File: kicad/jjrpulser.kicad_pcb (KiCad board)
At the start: 2 copper layers, 51.1 x 44.7 mm, 18 parts, among them J1 3.3V, J2 3.3V, J3 Screw_Terminal_HOT, J4 Screw_Terminal_COLD, J5 Conn_UART, U1 ESP-12

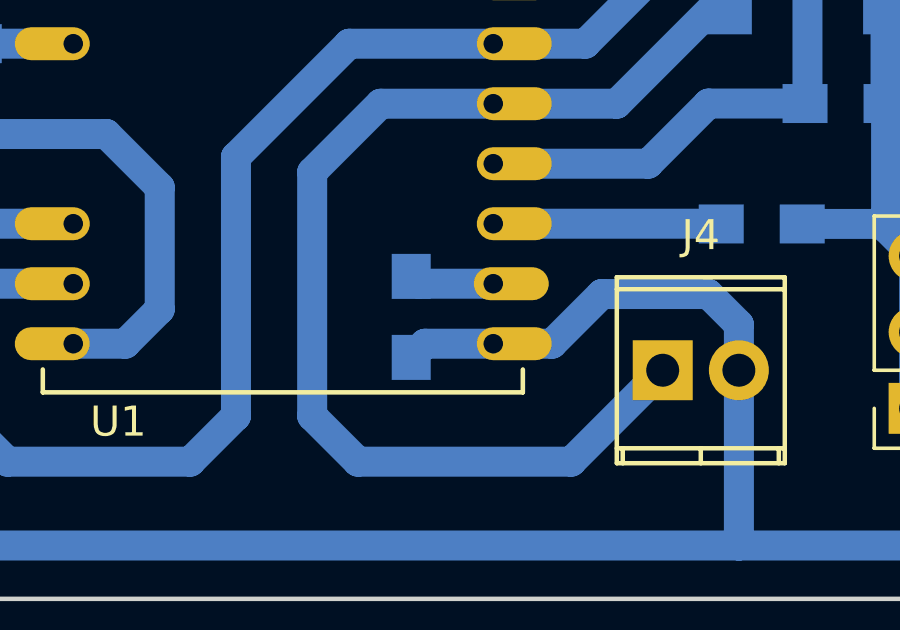
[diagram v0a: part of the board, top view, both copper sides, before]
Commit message: Еще немного гламура в трассировку
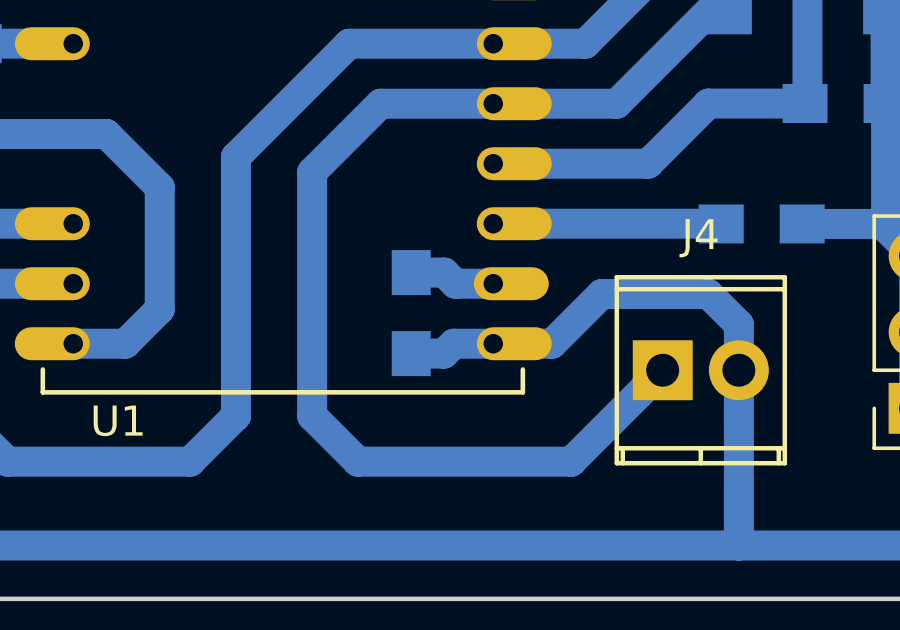
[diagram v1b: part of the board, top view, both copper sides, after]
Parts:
- moved R6 0.13 mm to (159.8, 118.0)
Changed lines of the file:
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@@
     (links 42)
     (no_connects 0)
-    (area 129.972999 81.272999 181.177001 127.583001)
+    (area 129.972999 82.728999 181.177001 127.583001)
     (thickness 1.6)
     (drawings 8)
-    (tracks 116)
+    (tracks 118)
     (zones 0)
     (modules 18)
@@
   )
   (module Resistors_SMD:R_0805_HandSoldering (layer B.Cu)
-    (at 159.766 118.11 90)
+    (at 159.766 117.983 90)
     (descr "Resistor SMD 0805, hand soldering")
     (tags "resistor 0805")
@@
   (gr_line (start 181.102 82.804) (end 181.102 127.508) (angle 90) (layer Edge.Cuts) (width 0.15))
   (gr_line (start 130.048 127.508) (end 130.048 82.804) (angle 90) (layer Edge.Cuts) (width 0.15))
+  (segment (start 162.5011 119.0036) (end 161.18586 119.0036) (width 1) (layer B.Cu) (net 1) (status 400000))
+  (segment (start 160.85646 119.333) (end 159.766 119.333) (width 1) (layer B.Cu) (net 1) (status 800000))
+  (segment (start 161.18586 119.0036) (end 160.85646 119.333) (width 1) (layer B.Cu) (net 1))
   (segment (start 134.62 116.078) (end 134.62 98.806) (width 1) (layer B.Cu) (net 1) (status 30))
   (segment (start 134.62 98.806) (end 134.62 96.266) (width 1) (layer B.Cu) (net 1) (status 10))
@@
   (segment (start 179.07 118.618) (end 179.07 121.158) (width 1) (layer B.Cu) (net 1) (status 30))
   (segment (start 170.688 125.73) (end 140.716 125.73) (width 1) (layer B.Cu) (net 1))
-  (segment (start 162.5011 119.0036) (end 160.2224 119.0036) (width 1) (layer B.Cu) (net 1) (status 30))
-  (segment (start 160.2224 119.0036) (end 159.766 119.46) (width 1) (layer B.Cu) (net 1) (status 30))
   (segment (start 139.954 98.806) (end 139.954 103.044) (width 1) (layer B.Cu) (net 2) (status 30))
   (segment (start 137.16 98.806) (end 137.16 103.044) (width 1) (layer B.Cu) (net 3) (status 30))
@@
   (segment (start 151.384 117.856) (end 151.384 113.792) (width 1) (layer B.Cu) (net 4))
   (segment (start 150.2364 119.0036) (end 151.384 117.856) (width 1) (layer B.Cu) (net 4))
-  (segment (start 162.5011 117.0036) (end 160.0096 117.0036) (width 1) (layer B.Cu) (net 5) (status 30))
-  (segment (start 160.0096 117.0036) (end 159.766 116.76) (width 1) (layer B.Cu) (net 5) (status 30))
+  (segment (start 162.5011 117.0036) (end 161.23896 117.0036) (width 1) (layer B.Cu) (net 5) (status 400000))
+  (segment (start 160.86836 116.633) (end 159.766 116.633) (width 1) (layer B.Cu) (net 5) (status 800000))
+  (segment (start 161.23896 117.0036) (end 160.86836 116.633) (width 1) (layer B.Cu) (net 5))
   (segment (start 162.5011 115.0036) (end 170.0924 115.0036) (width 1) (layer B.Cu) (net 6))
   (segment (start 162.5011 113.0036) (end 167.6664 113.0036) (width 1) (layer B.Cu) (net 7) (status 10))
